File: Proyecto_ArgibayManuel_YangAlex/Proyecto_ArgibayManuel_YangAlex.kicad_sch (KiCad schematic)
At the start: 23 parts, among them J1 Conn_01x04, J2 Conn_01x04, J3 Conn_01x06, SW1 SW_Push, SW2 SW_Push, SW3 SW_Push, SW4 SW_Push, U1 PIC18F258-I_SO, U2 LT1716IS5TRMPBF, U3 LT1716IS5TRMPBF, U7 HDC2010YPAR, Y1 Crystal

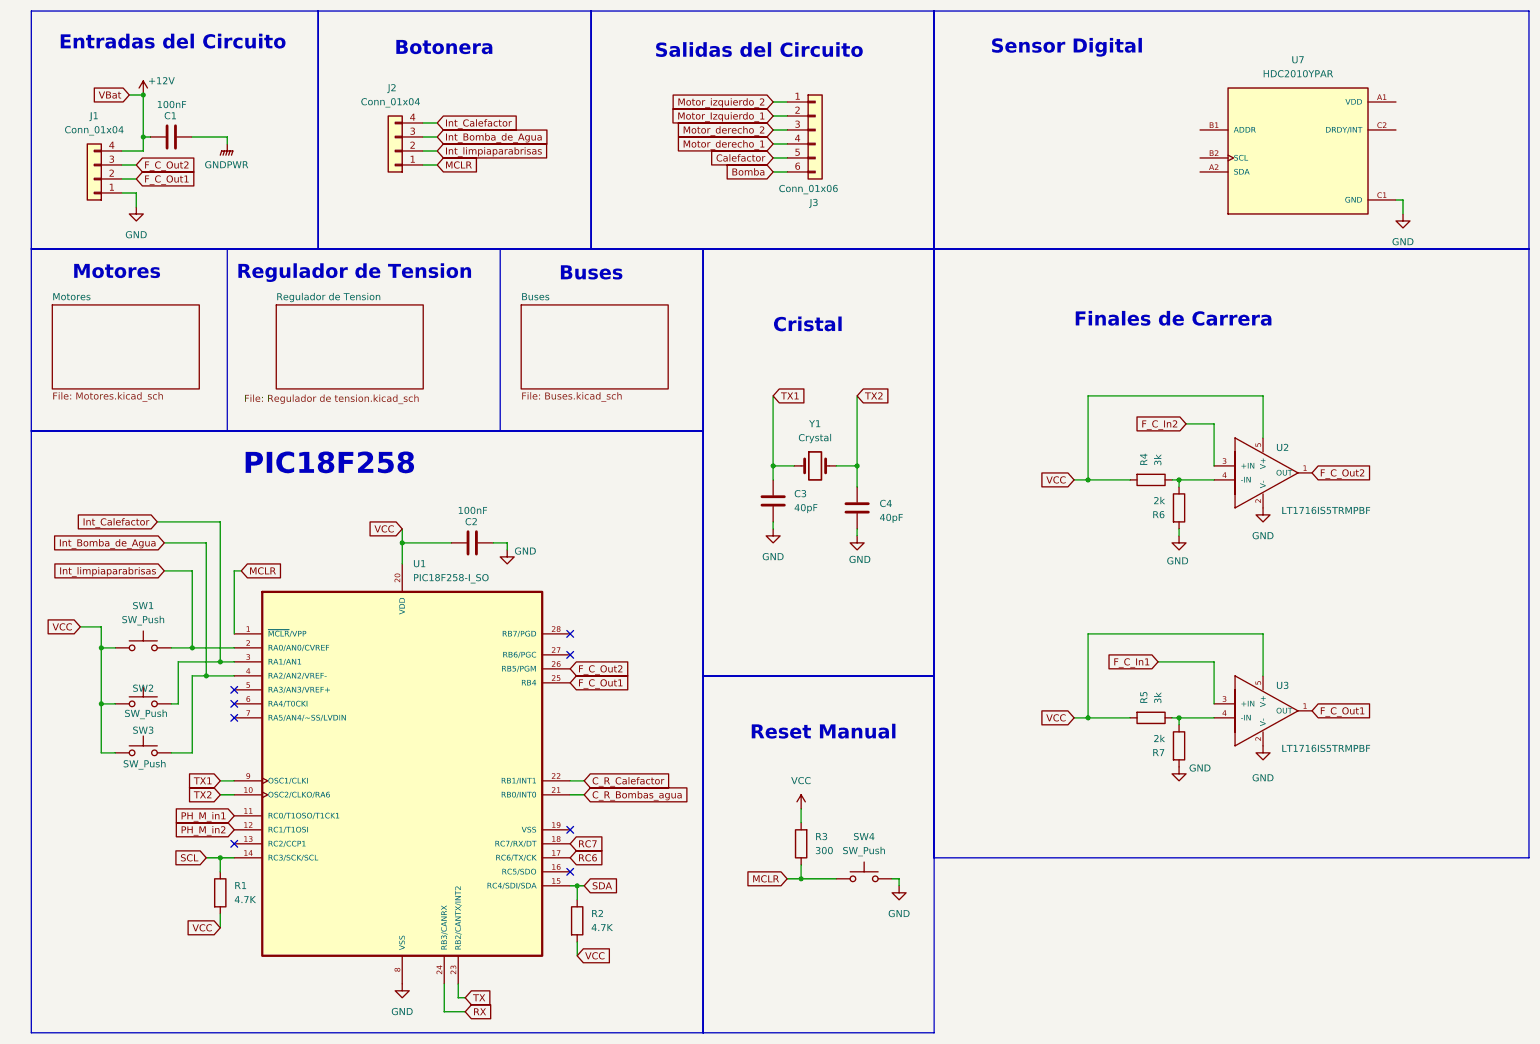
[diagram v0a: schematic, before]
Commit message: empezando a añadir el sensor(aun no esta terminado)
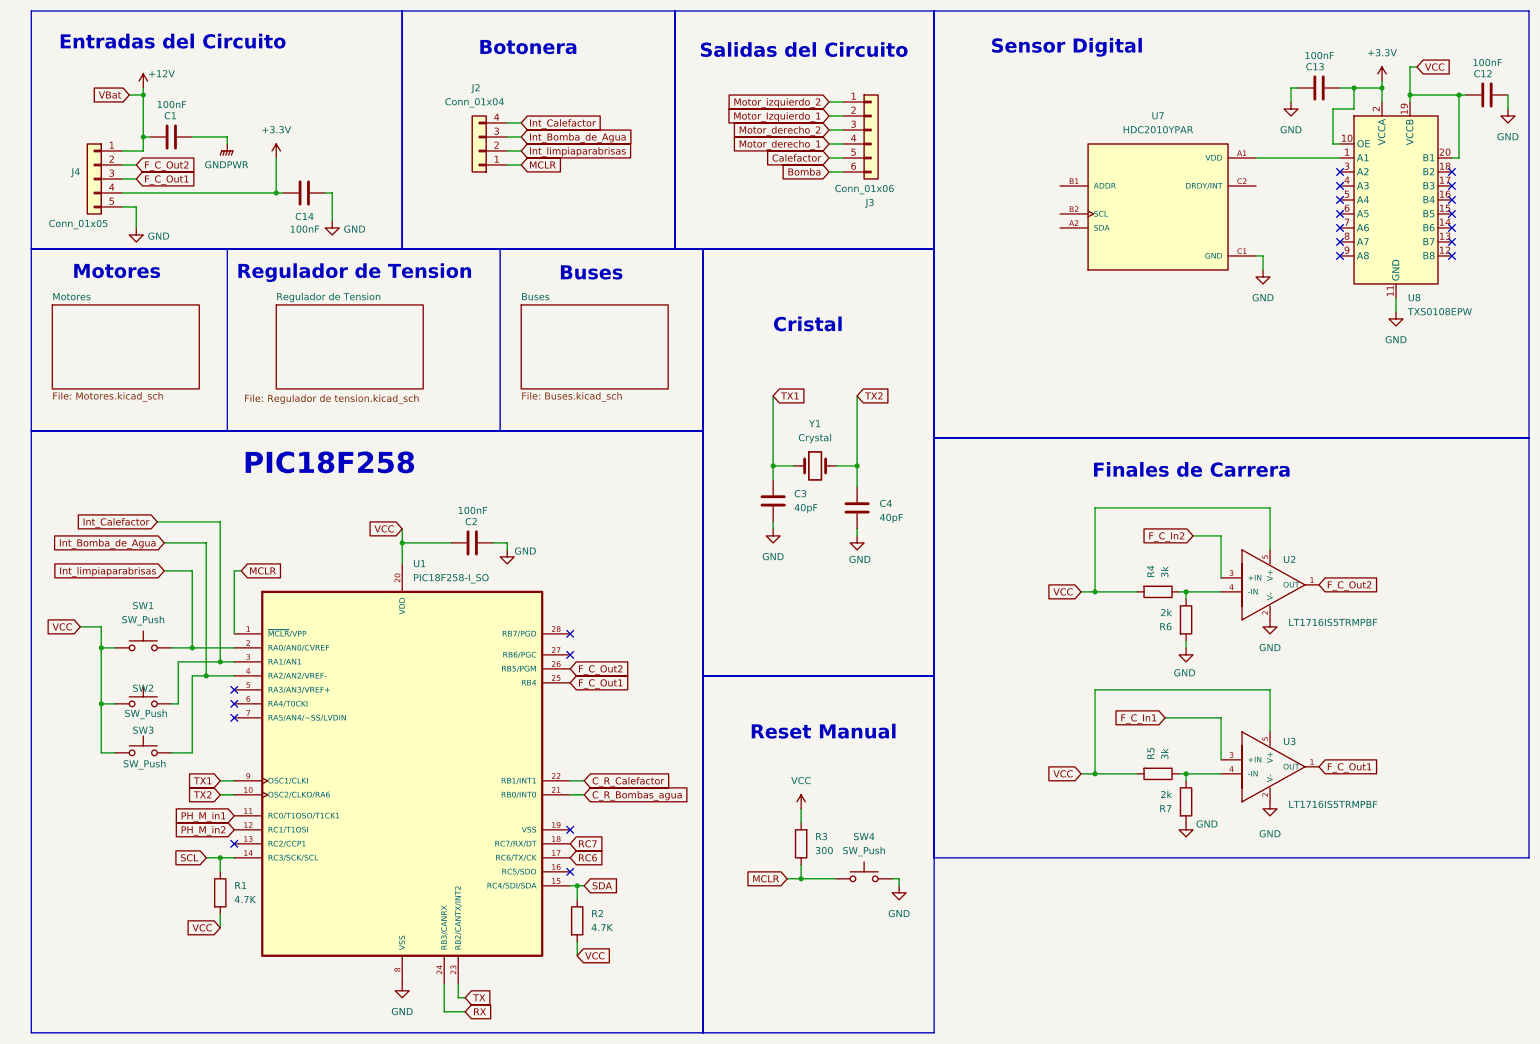
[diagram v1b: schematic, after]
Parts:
- removed J1: Conn_01x04, Connector_PinHeader_2.54mm:PinHeader_1x04_P2.54mm_Vertical, symbol Connector_Generic:Conn_01x04
- added C12, C13, C14: 100nF, Capacitor_SMD:C_0805_2012Metric, symbol Device:C
- added J4: Conn_01x05, symbol Connector_Generic:Conn_01x05
- added U8: TXS0108EPW, Package_SO:TSSOP-20_4.4x6.5mm_P0.65mm, symbol Logic_LevelTranslator:TXS0108EPW
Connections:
- net +12V: now also J4.1 (Pin_1)
- net F_C_Out1: now also J4.3 (Pin_3)
- net F_C_Out2: now also J4.2 (Pin_2)
- net GND: now also C12.2, C13.1, C14.2, J4.5 (Pin_5), U8.11 (GND)
- net VCC: now also C12.1, U8.19 (VCCB), U8.20 (B1)
- net at U7.A1 (VDD): now also U8.1 (A1)
- new net +3.3V: C13.2, C14.1, J4.4 (Pin_4), U8.10 (OE), U8.2 (VCCA)
- no-connect marks 8 -> 22
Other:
- moved on the sheet: J2, J3, R4, R5, R6, R7, U2, U3, U7

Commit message: sensor
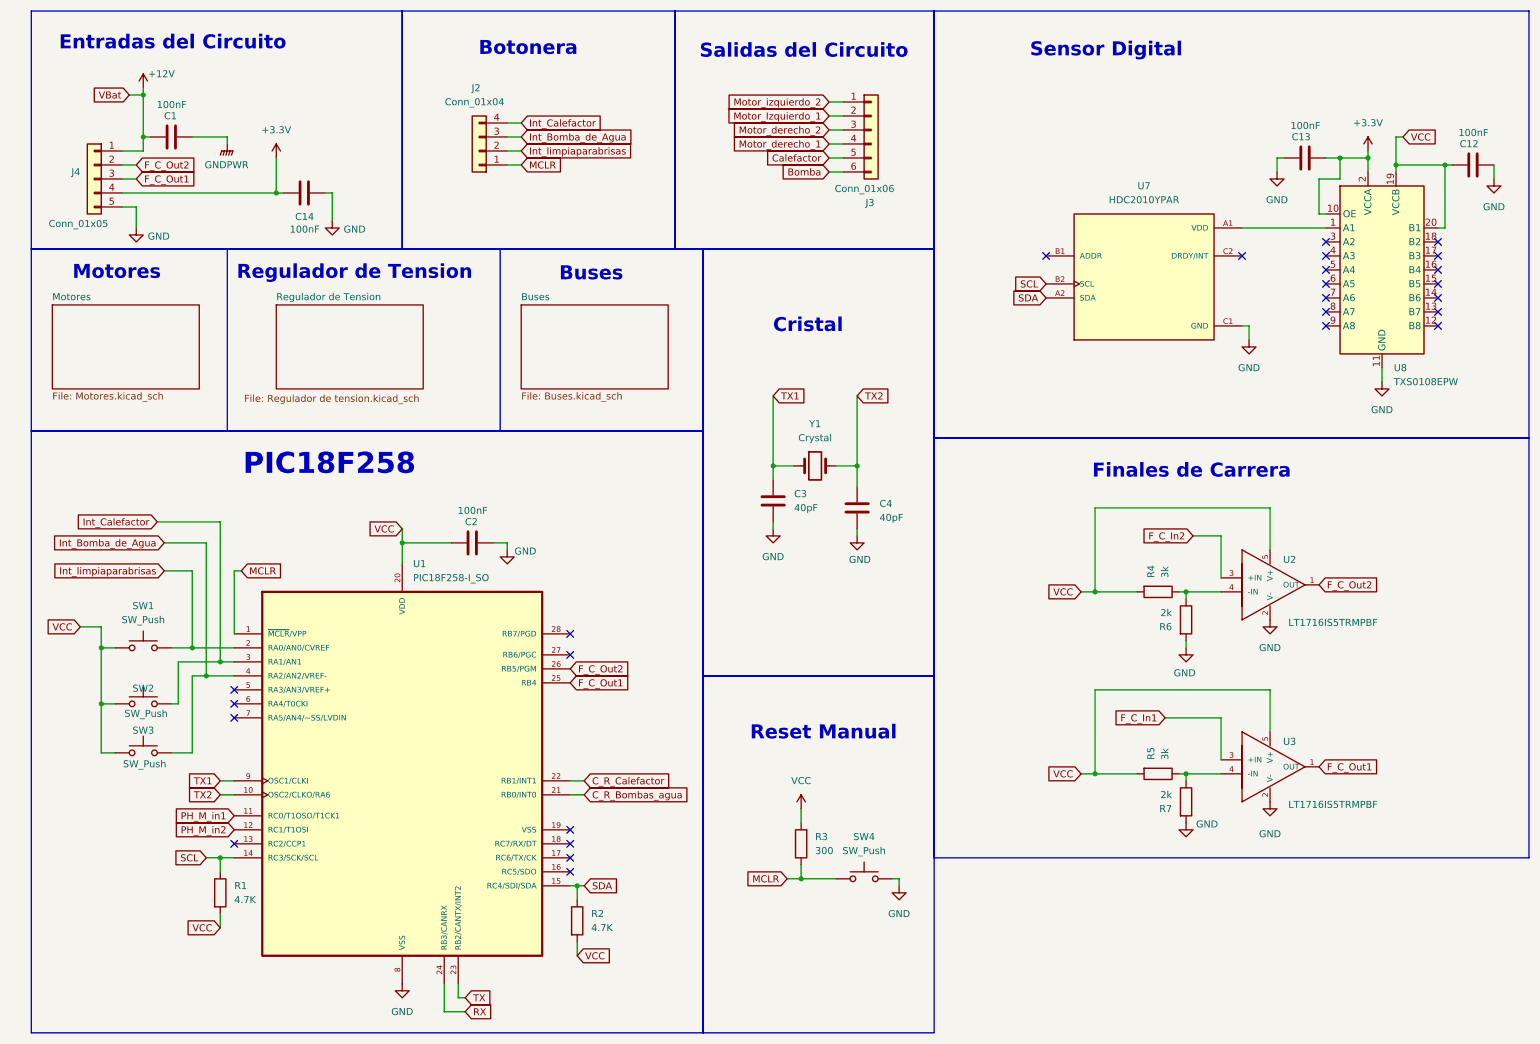
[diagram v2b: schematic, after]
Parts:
- J4: footprint (none) -> Connector_PinHeader_2.54mm:PinHeader_1x04_P2.54mm_Vertical
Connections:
- net SCL: now also U7.B2 (SCL)
- net SDA: now also U7.A2 (SDA)
- net RC6: no longer names the net of U1.17 (RC6/TX/CK)
- net RC7: no longer names the net of U1.18 (RC7/RX/DT)
- no-connect marks 22 -> 26
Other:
- moved on the sheet: C12, C13, U7, U8
